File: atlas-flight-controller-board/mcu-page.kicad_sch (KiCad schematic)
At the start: 1 part

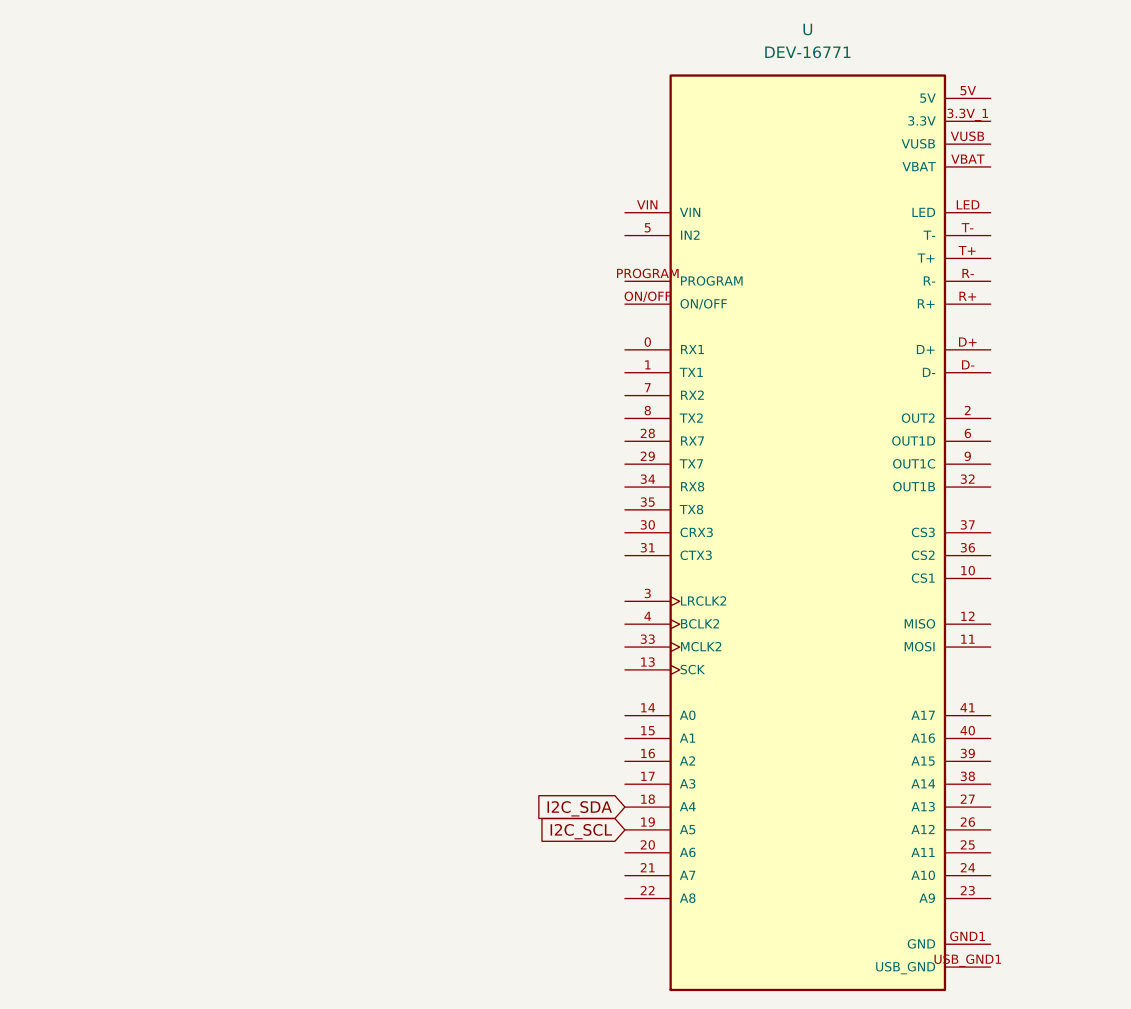
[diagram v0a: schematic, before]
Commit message: finishing up schematic for v1.
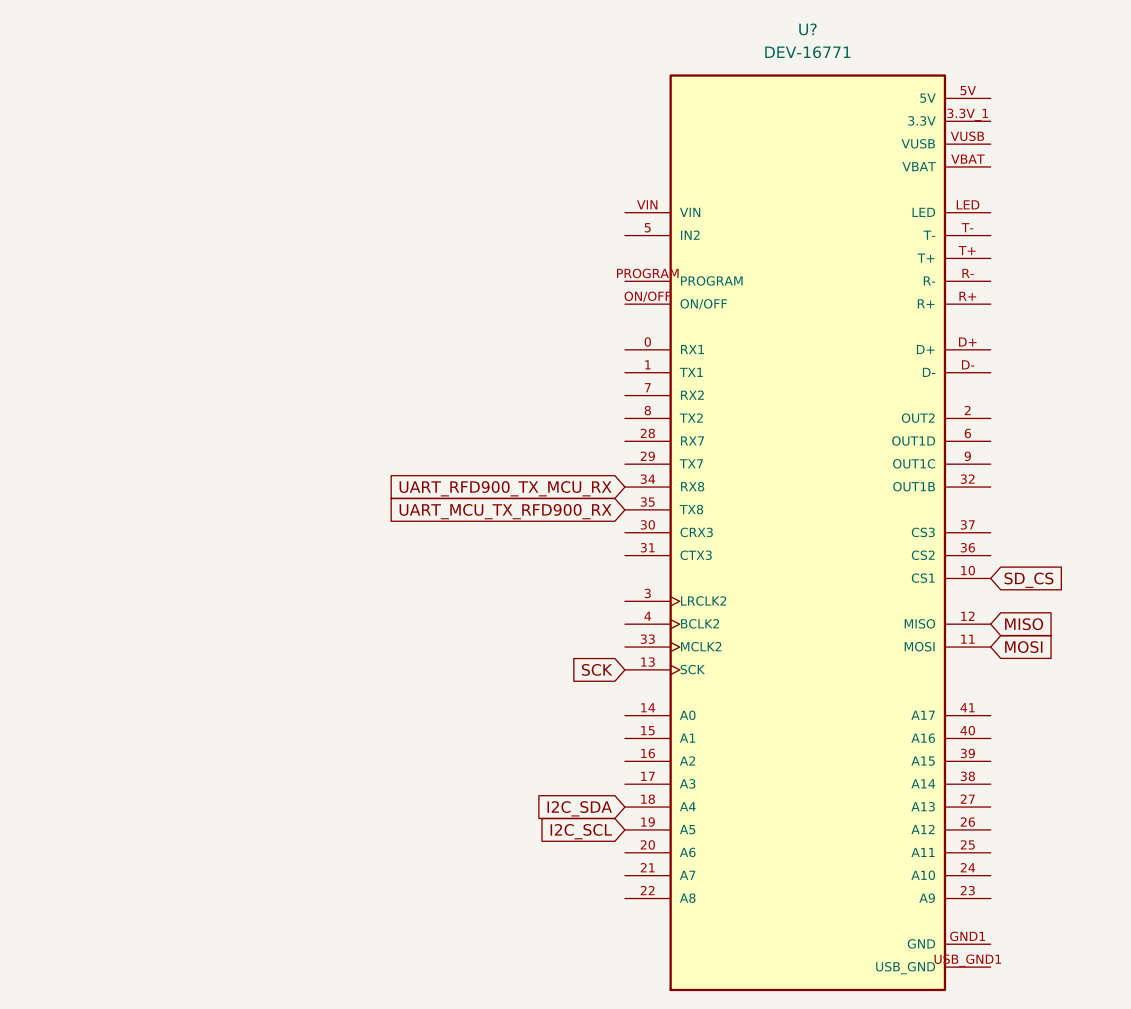
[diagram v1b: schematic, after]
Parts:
- renumbered U to U?
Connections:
- net SD_CS: now reaches U?.10 (CS1)
- net MOSI: now reaches U?.11 (MOSI)
- net MISO: now reaches U?.12 (MISO)
- net SCK: now reaches U?.13 (SCK)
- net UART_RFD900_TX_MCU_RX: now reaches U?.34 (RX8)
- net UART_MCU_TX_RFD900_RX: now reaches U?.35 (TX8)
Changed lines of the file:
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@@
 	(generator_version "9.0")
 	(paper "A4")
+	(global_label "UART_RFD900_TX_MCU_RX"
+		(shape input)
+		(at 124.46 83.82 180)
+		(fields_autoplaced yes)
+		(effects
+			(font
+				(size 1.27 1.27)
+			)
+			(justify right)
+		)
+		(property "Intersheetrefs" "${INTERSHEET_REFS}"
+			(at 96.9821 83.82 0)
+			(effects
+				(font
+					(size 1.27 1.27)
+				)
+				(justify right)
+				(hide yes)
+			)
+		)
+	)
+	(global_label "MOSI"
+		(shape input)
+		(at 165.1 101.6 0)
+		(fields_autoplaced yes)
+		(effects
+			(font
+				(size 1.27 1.27)
+			)
+			(justify left)
+		)
+		(property "Intersheetrefs" "${INTERSHEET_REFS}"
+			(at 172.6814 101.6 0)
+			(effects
+				(font
+					(size 1.27 1.27)
+				)
+				(justify left)
+				(hide yes)
+			)
+		)
+	)
 	(global_label "I2C_SDA"
 		(shape input)
@@
 		)
 	)
+	(global_label "UART_MCU_TX_RFD900_RX"
+		(shape input)
+		(at 124.46 86.36 180)
+		(fields_autoplaced yes)
+		(effects
+			(font
+				(size 1.27 1.27)
+			)
+			(justify right)
+		)
+		(property "Intersheetrefs" "${INTERSHEET_REFS}"
+			(at 96.9821 86.36 0)
+			(effects
+				(font
+					(size 1.27 1.27)
+				)
+				(justify right)
+				(hide yes)
+			)
+		)
+	)
 	(global_label "I2C_SCL"
 		(shape input)
@@
 				)
 				(justify right)
+				(hide yes)
+			)
+		)
+	)
+	(global_label "SCK"
+		(shape input)
+		(at 124.46 104.14 180)
+		(fields_autoplaced yes)
+		(effects
+			(font
+				(size 1.27 1.27)
+			)
+			(justify right)
+		)
+		(property "Intersheetrefs" "${INTERSHEET_REFS}"
+			(at 117.7253 104.14 0)
+			(effects
+				(font
+					(size 1.27 1.27)
+				)
+				(justify right)
+				(hide yes)
+			)
+		)
+	)
+	(global_label "MISO"
+		(shape input)
+		(at 165.1 99.06 0)
+		(fields_autoplaced yes)
+		(effects
+			(font
+				(size 1.27 1.27)
+			)
+			(justify left)
+		)
+		(property "Intersheetrefs" "${INTERSHEET_REFS}"
+			(at 172.6814 99.06 0)
+			(effects
+				(font
+					(size 1.27 1.27)
+				)
+				(justify left)
+				(hide yes)
+			)
+		)
+	)
+	(global_label "SD_CS"
+		(shape input)
+		(at 165.1 93.98 0)
+		(fields_autoplaced yes)
+		(effects
+			(font
+				(size 1.27 1.27)
+			)
+			(justify left)
+		)
+		(property "Intersheetrefs" "${INTERSHEET_REFS}"
+			(at 174.0118 93.98 0)
+			(effects
+				(font
+					(size 1.27 1.27)
+				)
+				(justify left)
 				(hide yes)
 			)
@@
 		(dnp no)
 		(fields_autoplaced yes)
-		(property "Reference" "U"
+		(property "Reference" "U?"
 			(at 144.78 33.02 0)
 			(effects
@@
 		(instances
 			(project "atlas-flight-controller-board"
-				(path "/99efb2d6-b5f7-438c-9ed2-f359400f01a1/0e8824f2-4013-4596-998b-cdfa7c1cf328"
-					(reference "U3")
+				(path "/99efb2d6-b5f7-438c-9ed2-f359400f01a1/ebeff960-adac-492b-ba2d-f8a8dedd6bc1"
+					(reference "U?")
 					(unit 1)
 				)

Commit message: wip commit
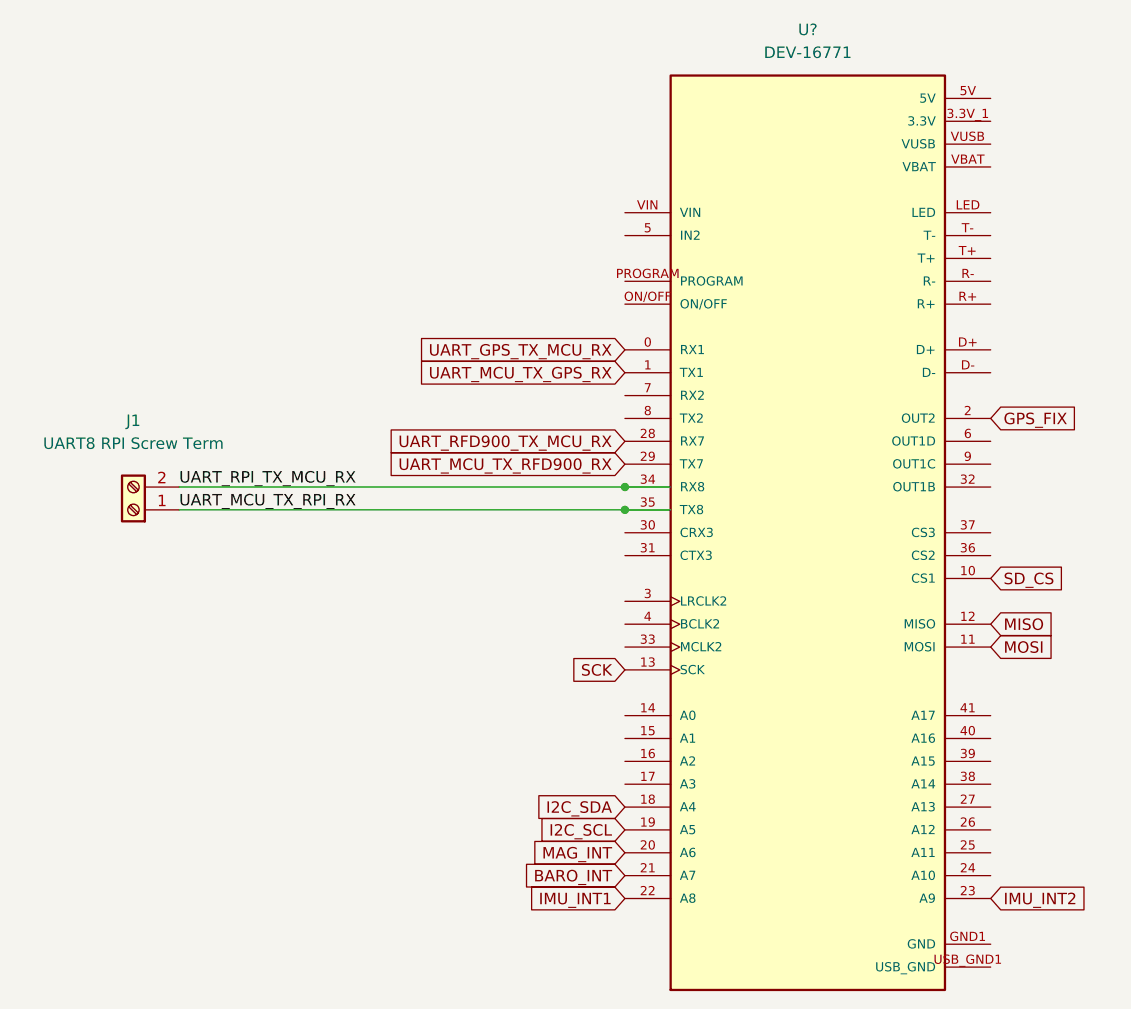
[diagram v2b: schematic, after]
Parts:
- added J1: UART8 RPI Screw Term, TerminalBlock:TerminalBlock_Xinya_XY308-2.54-2P_1x02_P2.54mm_Horizontal, symbol Connector:Screw_Terminal_01x02
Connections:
- net UART_MCU_TX_RFD900_RX: now also U?.29 (TX7); no longer U?.35 (TX8)
- net UART_RFD900_TX_MCU_RX: now also U?.28 (RX7); no longer U?.34 (RX8)
- net UART_GPS_TX_MCU_RX: now reaches U?.0 (RX1)
- net UART_MCU_TX_GPS_RX: now reaches U?.1 (TX1)
- net GPS_FIX: now reaches U?.2 (OUT2)
- net MAG_INT: now reaches U?.20 (A6)
- net BARO_INT: now reaches U?.21 (A7)
- net IMU_INT1: now reaches U?.22 (A8)
- net IMU_INT2: now reaches U?.23 (A9)
- new net UART_MCU_TX_RPI_RX: J1.1 (Pin_1), U?.35 (TX8)
- new net UART_RPI_TX_MCU_RX: J1.2 (Pin_2), U?.34 (RX8)
